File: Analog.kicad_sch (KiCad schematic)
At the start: 24 parts, among them Q2 2N7002, U3 74HC4051, U4 74HC4051, U5 OPA350, U6 MAX5423

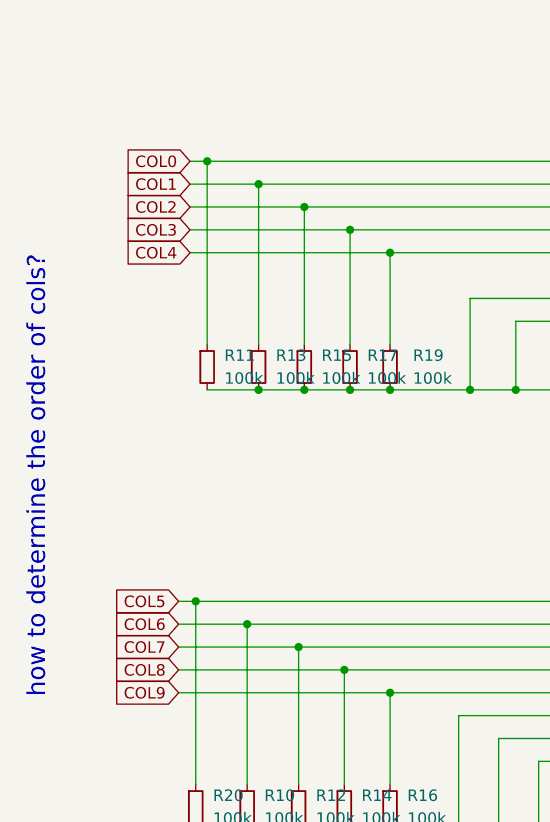
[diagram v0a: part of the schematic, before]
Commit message: routing work
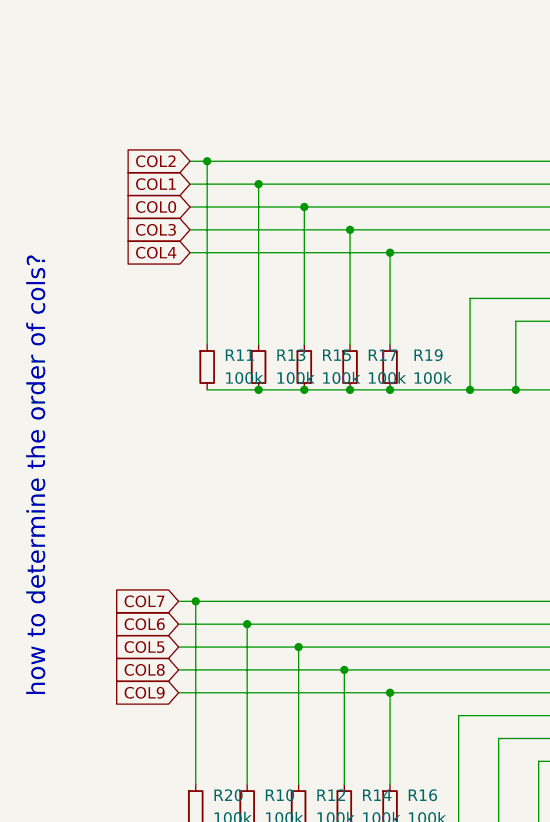
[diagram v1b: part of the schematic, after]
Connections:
- net COL0: now also R15.1, U4.15 (A2); no longer R11.1, U4.13 (A0)
- net COL2: now also R11.1, U4.13 (A0); no longer R15.1, U4.15 (A2)
- net COL5: now also R12.1, U3.15 (A2); no longer R20.1, U3.13 (A0)
- net COL7: now also R20.1, U3.13 (A0); no longer R12.1, U3.15 (A2)
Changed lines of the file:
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@@
     )
   )
-  (global_label "COL2" (shape input) (at 67.945 47.625 180) (fields_autoplaced)
+  (global_label "COL2" (shape input) (at 67.945 42.545 180) (fields_autoplaced)
     (effects (font (size 1.27 1.27)) (justify right))
-    (property "Intersheet References" "${INTERSHEET_REFS}" (id 0) (at 60.6938 47.7044 0)
+    (property "Intersheet References" "${INTERSHEET_REFS}" (id 0) (at 60.6938 42.6244 0)
       (effects (font (size 1.27 1.27)) (justify right) hide)
     )
@@
     )
   )
-  (global_label "COL7" (shape input) (at 66.675 96.52 180) (fields_autoplaced)
+  (global_label "COL7" (shape input) (at 66.675 91.44 180) (fields_autoplaced)
     (effects (font (size 1.27 1.27)) (justify right))
-    (property "Intersheet References" "${INTERSHEET_REFS}" (id 0) (at 59.4238 96.5994 0)
+    (property "Intersheet References" "${INTERSHEET_REFS}" (id 0) (at 59.4238 91.5194 0)
       (effects (font (size 1.27 1.27)) (justify right) hide)
     )
@@
     )
   )
-  (global_label "COL0" (shape input) (at 67.945 42.545 180) (fields_autoplaced)
+  (global_label "COL0" (shape input) (at 67.945 47.625 180) (fields_autoplaced)
     (effects (font (size 1.27 1.27)) (justify right))
-    (property "Intersheet References" "${INTERSHEET_REFS}" (id 0) (at 60.6938 42.6244 0)
+    (property "Intersheet References" "${INTERSHEET_REFS}" (id 0) (at 60.6938 47.7044 0)
       (effects (font (size 1.27 1.27)) (justify right) hide)
     )
@@
     )
   )
-  (global_label "COL5" (shape input) (at 66.675 91.44 180) (fields_autoplaced)
+  (global_label "COL5" (shape input) (at 66.675 96.52 180) (fields_autoplaced)
     (effects (font (size 1.27 1.27)) (justify right))
-    (property "Intersheet References" "${INTERSHEET_REFS}" (id 0) (at 59.4238 91.5194 0)
+    (property "Intersheet References" "${INTERSHEET_REFS}" (id 0) (at 59.4238 96.5994 0)
       (effects (font (size 1.27 1.27)) (justify right) hide)
     )
